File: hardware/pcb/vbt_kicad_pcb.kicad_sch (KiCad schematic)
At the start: 0 parts

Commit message: Updated v2 schematics
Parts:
- added BT1: Battery, symbol Device:Battery
- added U1: ESP32-WROOM-32E, RF_Module:ESP32-WROOM-32E, symbol RF_Module:ESP32-WROOM-32E

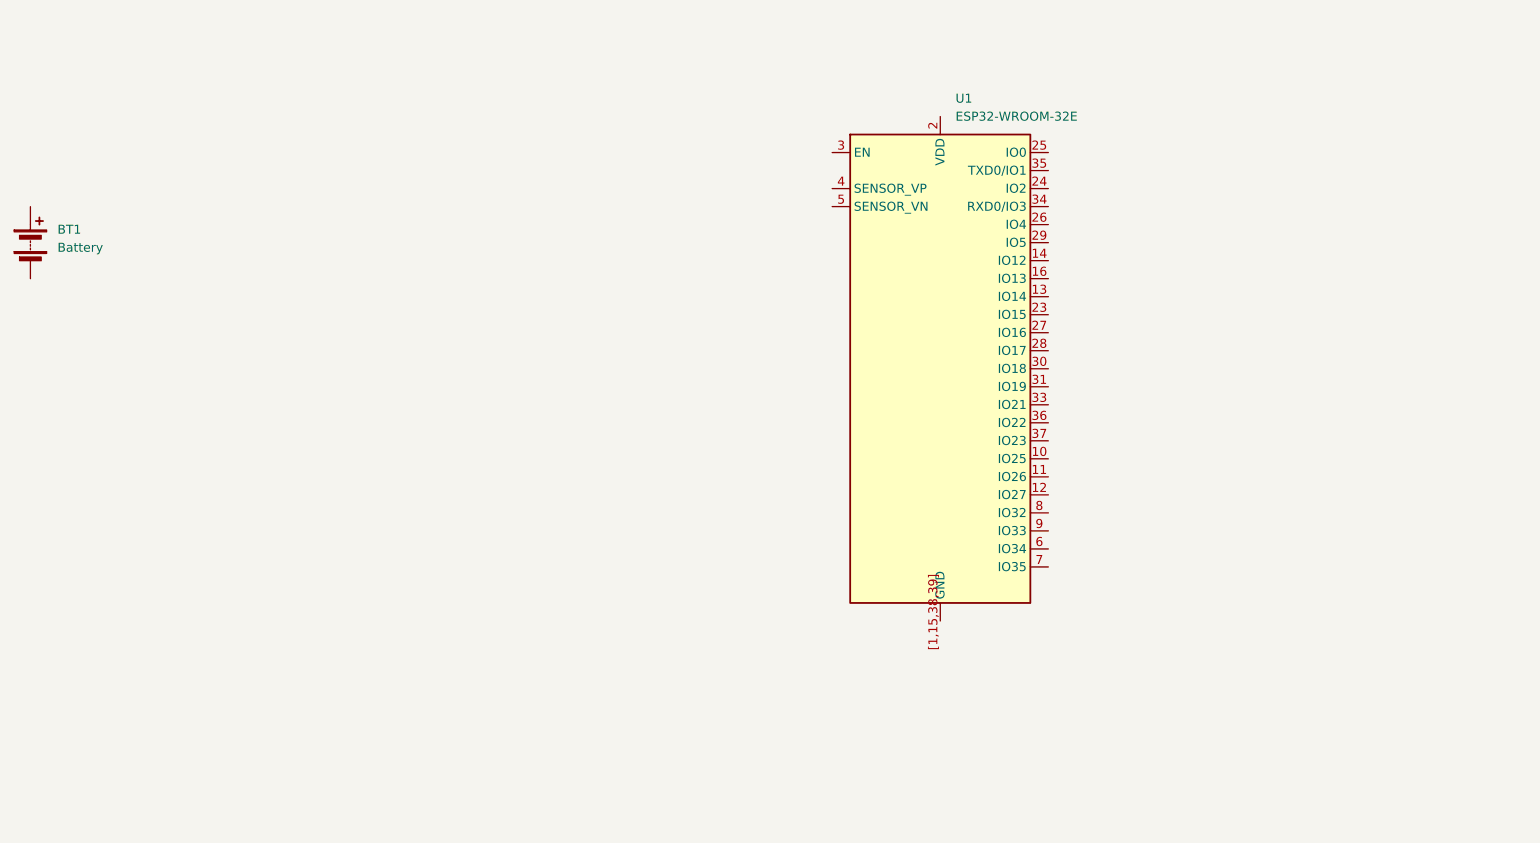
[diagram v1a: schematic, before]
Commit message: Add KiCad rev A project
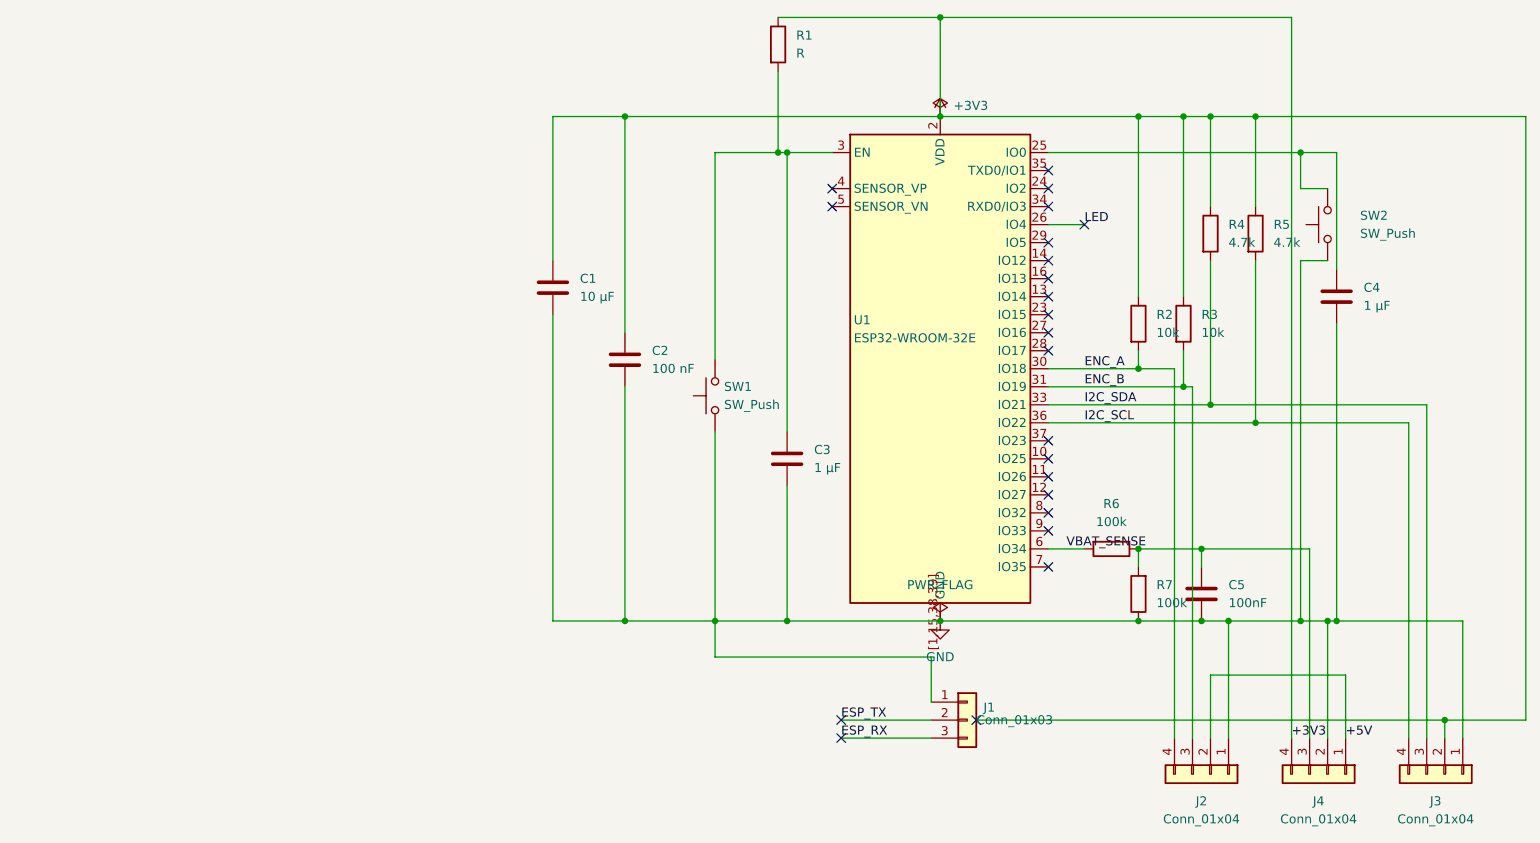
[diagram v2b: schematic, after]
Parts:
- removed BT1: Battery, symbol Device:Battery
- added C1: 10 µF, Capacitor_SMD:C_0805_2012Metric, symbol Device:C
- added C2: 100 nF, Capacitor_SMD:C_0805_2012Metric, symbol Device:C
- added C3, C4: 1 µF, Capacitor_SMD:C_0805_2012Metric, symbol Device:C
- added C5: 100nF, symbol Device:C
- added J1: Conn_01x03, Connector_PinSocket_2.54mm:PinSocket_1x03_P2.54mm_Vertical, symbol Connector_Generic:Conn_01x03
- added J2, J3, J4: Conn_01x04, Connector:FanPinHeader_1x04_P2.54mm_Vertical, symbol Connector_Generic:Conn_01x04
- added R1: R, Resistor_SMD:R_0805_2012Metric, symbol Device:R
- added R2, R3: 10k, Resistor_SMD:R_0805_2012Metric, symbol Device:R
- added R4, R5: 4.7k, Resistor_SMD:R_0805_2012Metric, symbol Device:R
- added R6, R7: 100k, Resistor_SMD:R_0805_2012Metric_Pad1.20x1.40mm_HandSolder, symbol Device:R
- added SW1, SW2: SW_Push, Inductor_SMD:L_0805_2012Metric, symbol Switch:SW_Push
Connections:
- net +3V3: now reaches U1.2 (VDD)
- net +3V3: now also C1.1, C2.1, J3.2 (Pin_2), J4.4 (Pin_4), R1.1, R2.1, R3.1, R4.1, R5.1
- net at U1.25 (IO0): now also C4.1, SW2.2
- net LED: now reaches U1.26 (IO4)
- net at U1.3 (EN): now also C3.1, R1.2, SW1.2
- net ENC_A: now reaches U1.30 (IO18)
- net ENC_A: now also J2.4 (Pin_4), R2.2
- net ENC_B: now reaches U1.31 (IO19)
- net ENC_B: now also J2.3 (Pin_3), R3.2
- net I2C_SDA: now reaches U1.33 (IO21)
- net I2C_SDA: now also J3.3 (Pin_3), R4.2
- net I2C_SCL: now reaches U1.36 (IO22)
- net I2C_SCL: now also J3.4 (Pin_4), R5.2
- net VBAT_SENSE: now reaches U1.6 (IO34)
- net VBAT_SENSE: now also R6.2
- net GND: now reaches U1.[1,15,38,39] (GND)
- net GND: now also C1.2, C2.2, C3.2, C4.2, C5.2, J1.1 (Pin_1), J2.1 (Pin_1), J3.1 (Pin_1), J4.2 (Pin_2), R7.1, SW1.1, SW2.1
- new net: C5.1, J4.3 (Pin_3), R6.1, R7.2
- new net +5V: J2.2 (Pin_2), J4.1 (Pin_1)
- new net ESP_RX: J1.3 (Pin_3)
- new net ESP_TX: J1.2 (Pin_2)
- no-connect marks 0 -> 23
